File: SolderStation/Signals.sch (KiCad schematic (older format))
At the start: 9 parts

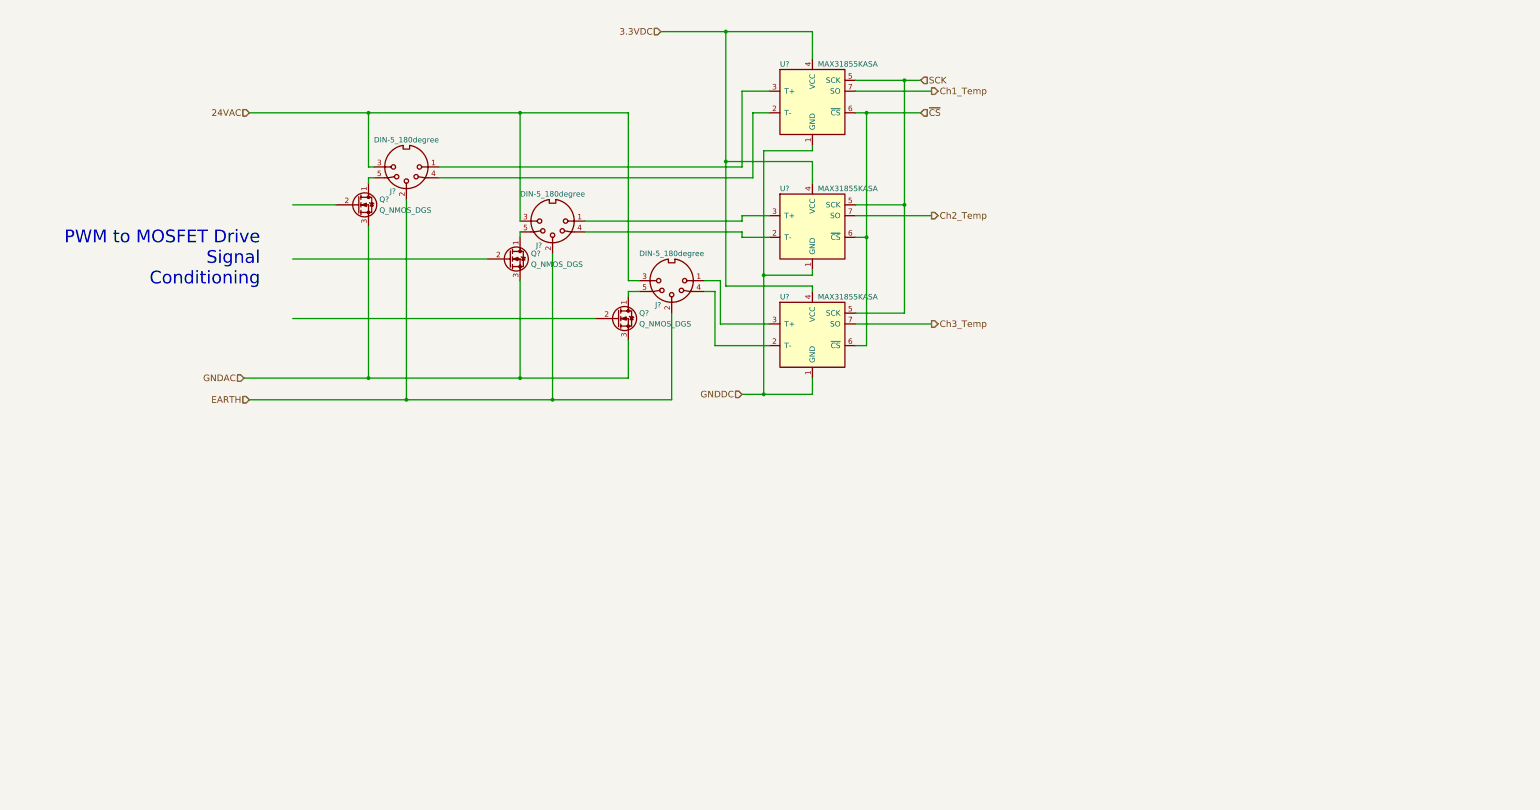
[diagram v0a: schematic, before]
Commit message: Revert "Add files via upload"
This reverts commit 9e82852e4677a33747f2b205dd1fce6c4e717f3a.
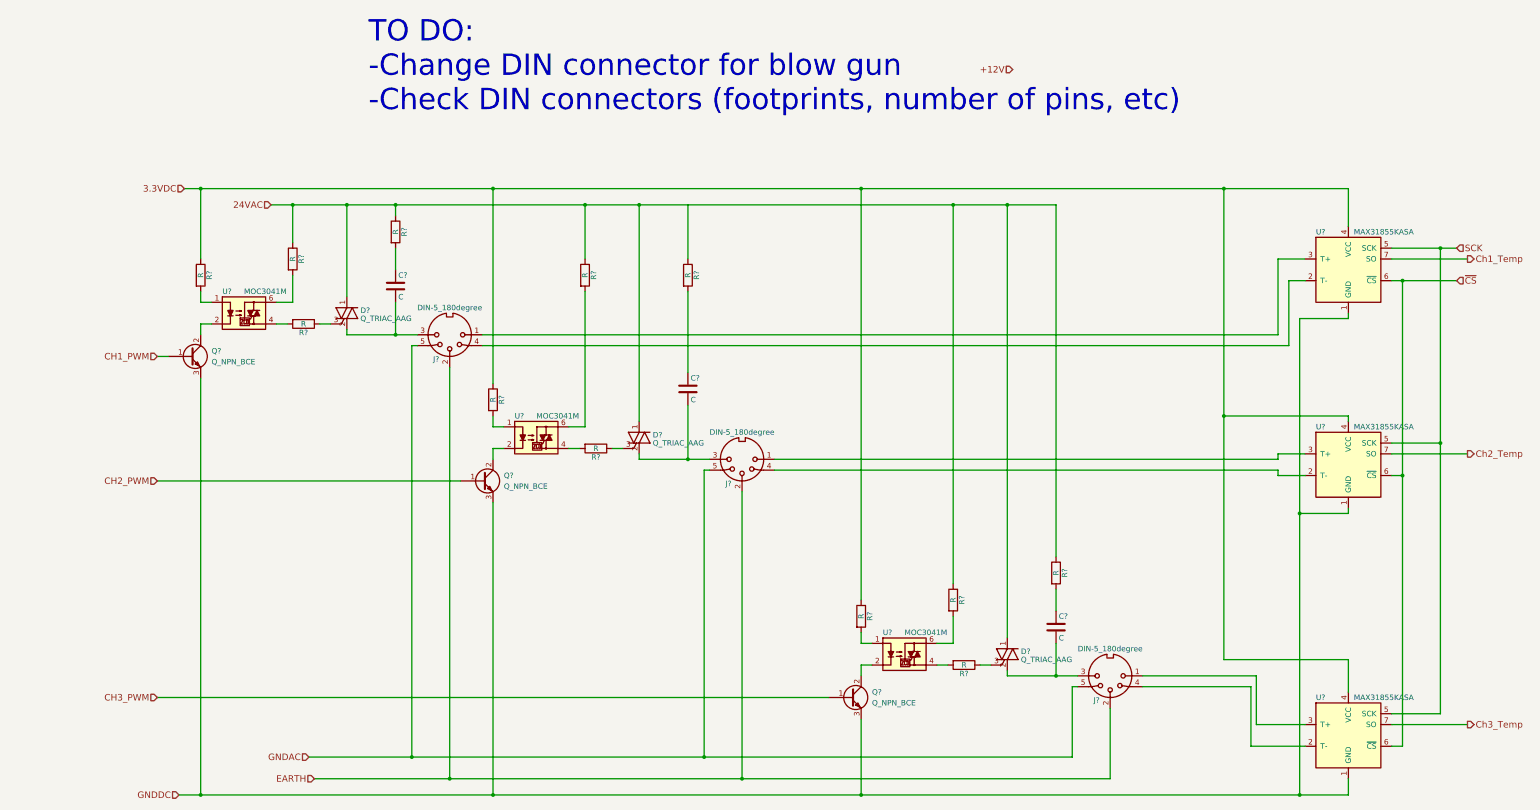
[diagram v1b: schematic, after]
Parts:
- removed J? (x2): DIN-5_180degree, symbol DIN-5_180degree
- removed Q? (x3): Q_NMOS_DGS, symbol Q_NMOS_DGS
- added C? (x3): C, symbol C
- added D? (x3): Q_TRIAC_AAG, symbol Q_TRIAC_AAG
- added J? (x2): DIN-5_180degree, symbol DIN-5_180degree
- added Q? (x3): Q_NPN_BCE, symbol Q_NPN_BCE
- added R? (x12): R, symbol R
- added U? (x3): MOC3041M, symbol MOC3041M
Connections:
- net labels added: +12V, CH1_PWM, CH2_PWM, CH3_PWM
- wire segments 80 -> 137
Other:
- note added: "TO DO:\n-Change DIN connector for blow gun\n-Check DIN connectors (footprints, number of pins, etc)\n"
- note removed: "PWM to MOSFET Drive\nSignal\nConditioning"
- moved on the sheet: J?, U?
